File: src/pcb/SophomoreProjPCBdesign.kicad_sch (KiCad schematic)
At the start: 22 parts, among them J1 AudioJack2, J2 AudioJack2, Q1 NJFET, SW1 SW_SPST, SW2 SW_SPST, U1 LM386

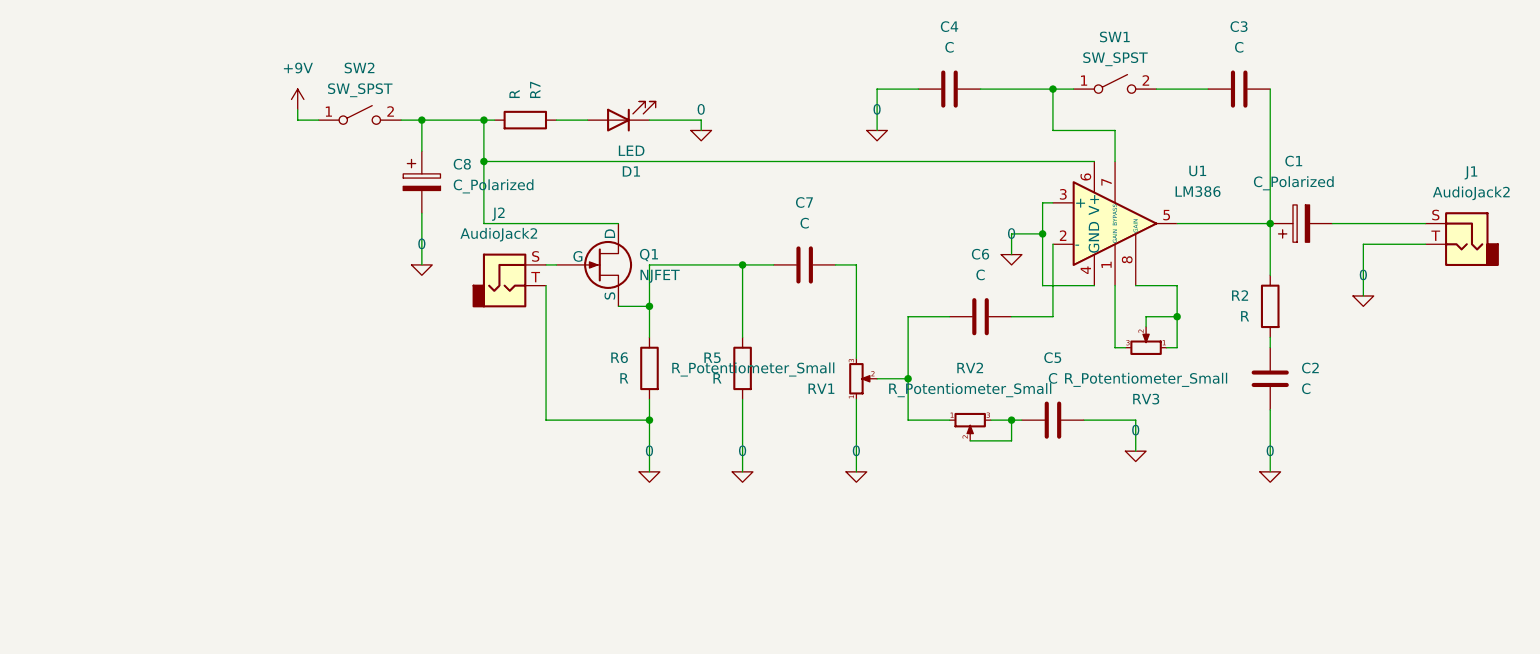
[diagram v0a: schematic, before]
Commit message: pcb: finalized pcb design
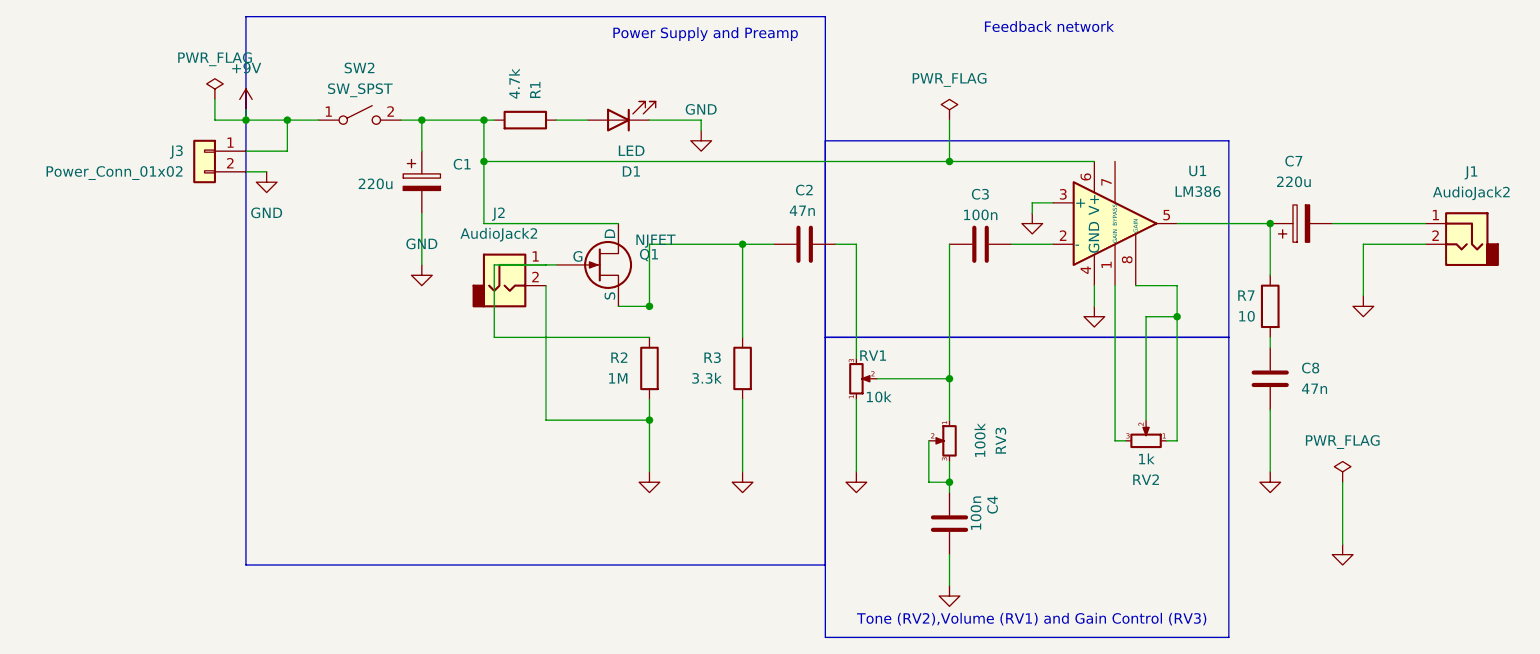
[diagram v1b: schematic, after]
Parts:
- removed C3, C4: C, symbol Device:C
- removed SW1: SW_SPST, symbol Switch:SW_SPST
- added J3: Power_Conn_01x02, Connector_PinHeader_2.54mm:PinHeader_2x01_P2.54mm_Vertical, symbol Connector_Generic:Conn_01x02
- C1: renamed from C8; value C_Polarized -> 220u; footprint (none) -> Capacitor_THT:CP_Radial_D8.0mm_P3.50mm
- C2: renamed from C7; value C -> 47n; footprint (none) -> Capacitor_THT:C_Disc_D5.0mm_W2.5mm_P5.00mm
- C3: renamed from C6; value C -> 100n; footprint (none) -> Capacitor_THT:C_Disc_D5.0mm_W2.5mm_P5.00mm
- C4: renamed from C5; value C -> 100n; footprint (none) -> Capacitor_THT:C_Disc_D5.0mm_W2.5mm_P5.00mm
- C7: renamed from C1; value C_Polarized -> 220u; footprint (none) -> Capacitor_THT:CP_Radial_D8.0mm_P3.50mm
- C8: renamed from C2; value C -> 47n; footprint (none) -> Capacitor_THT:C_Disc_D5.0mm_W2.5mm_P5.00mm
- D1: footprint (none) -> LED_THT:LED_D5.0mm
- J1, J2, SW2: footprint (none) -> Connector_PinHeader_2.54mm:PinHeader_1x02_P2.54mm_Vertical
- Q1: footprint (none) -> Package_TO_SOT_THT:TO-92_Inline
- R1: renamed from R7; value R -> 4.7k; footprint (none) -> Resistor_THT:R_Axial_DIN0207_L6.3mm_D2.5mm_P10.16mm_Horizontal
- R2: renamed from R6; value R -> 1M; footprint (none) -> Resistor_THT:R_Axial_DIN0207_L6.3mm_D2.5mm_P10.16mm_Horizontal
- R3: renamed from R5; value R -> 3.3k; footprint (none) -> Resistor_THT:R_Axial_DIN0207_L6.3mm_D2.5mm_P10.16mm_Horizontal
- R7: renamed from R2; value R -> 10; footprint (none) -> Resistor_THT:R_Axial_DIN0207_L6.3mm_D2.5mm_P10.16mm_Horizontal
- RV1: value R_Potentiometer_Small -> 10k; footprint (none) -> Potentiometer_THT:Potentiometer_Alpha_RD901F-40-00D_Single_Vertical
- RV2: renamed from RV3; value R_Potentiometer_Small -> 1k; footprint (none) -> Potentiometer_THT:Potentiometer_Alpha_RD901F-40-00D_Single_Vertical
- RV3: renamed from RV2; value R_Potentiometer_Small -> 100k; footprint (none) -> Potentiometer_THT:Potentiometer_Alpha_RD901F-40-00D_Single_Vertical
- U1: footprint (none) -> Package_SO:SOIC-8_3.9x4.9mm_P1.27mm
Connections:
- net +9V: now also J3.1 (Pin_1)
- net at Q1.2 (G): now also J2.1, R2.1; no longer J2.S
- net at C7.2: now also J1.1; no longer J1.S
- net at C2.2, Q1.3 (S), R3.1: no longer R2.1
- net 0 renamed GND
- net GND: now also J1.2, J2.2, J3.2 (Pin_2); no longer J1.T, J2.T
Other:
- note added: "Feedback network"
- note added: "Power Supply and Preamp"
- note added: "Tone (RV2),Volume (RV1) and Gain Control (RV3)"
- moved on the sheet: C2, C3, C4, RV2, RV3
